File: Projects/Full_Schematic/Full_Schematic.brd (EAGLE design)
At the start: 100 x 69 mm, 79 parts, among them J1 10118193-0001LF, Q1 SS8050-G, Q2 SS8050-G, SW1 OS102011MS2QN1, SW2 OS102011MS2QN1, U1 LM324, U10 SC189ZSKTRT, U2 ACS70331EESATR-005U3, U3 74HC4051PW,118, U4 NA555DR, U5 FT260Q-T, U6 MIC5387-SGFYMT-TR, U7 ESP32-WROOM-32E_(16MB), U8 SCD41-D-R1, U9 HDC1080DMBR

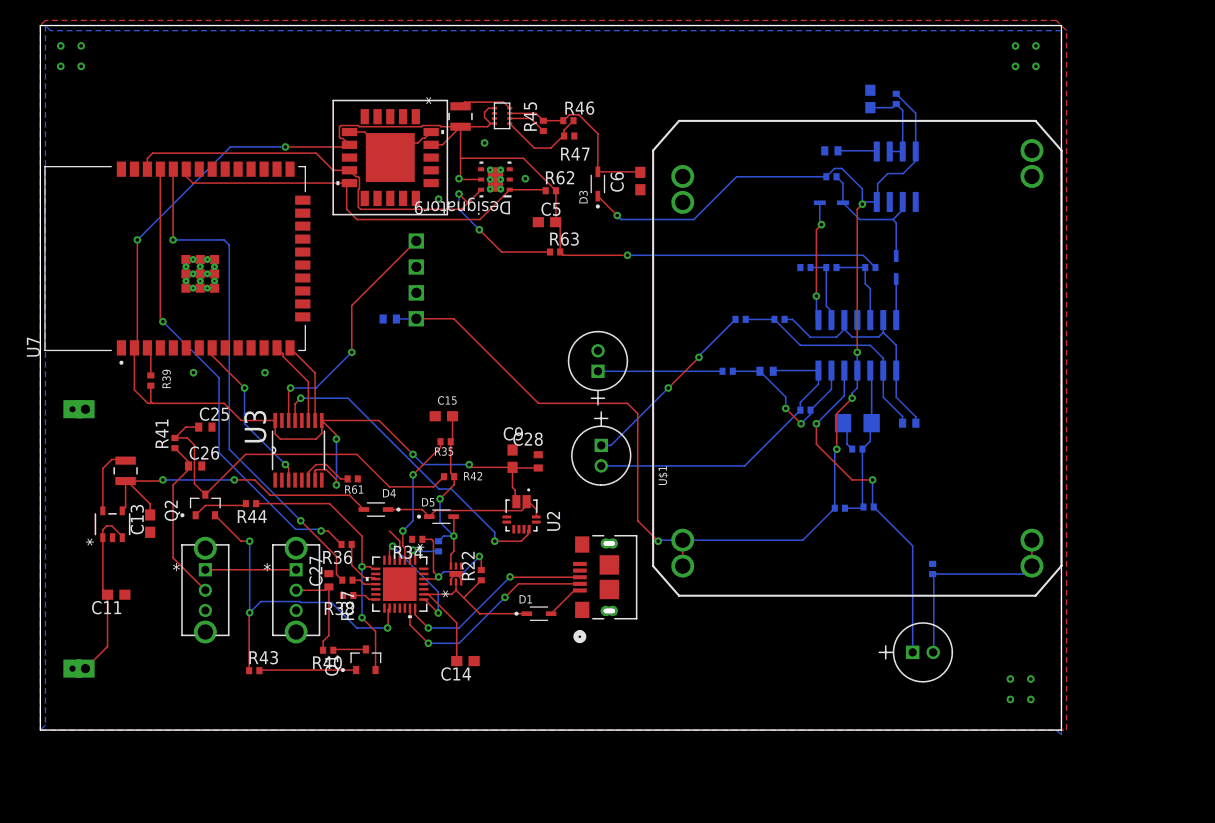
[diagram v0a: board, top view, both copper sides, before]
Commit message: Final revision of the Full Schematic, haven't updated in a while since I was soloing this one.
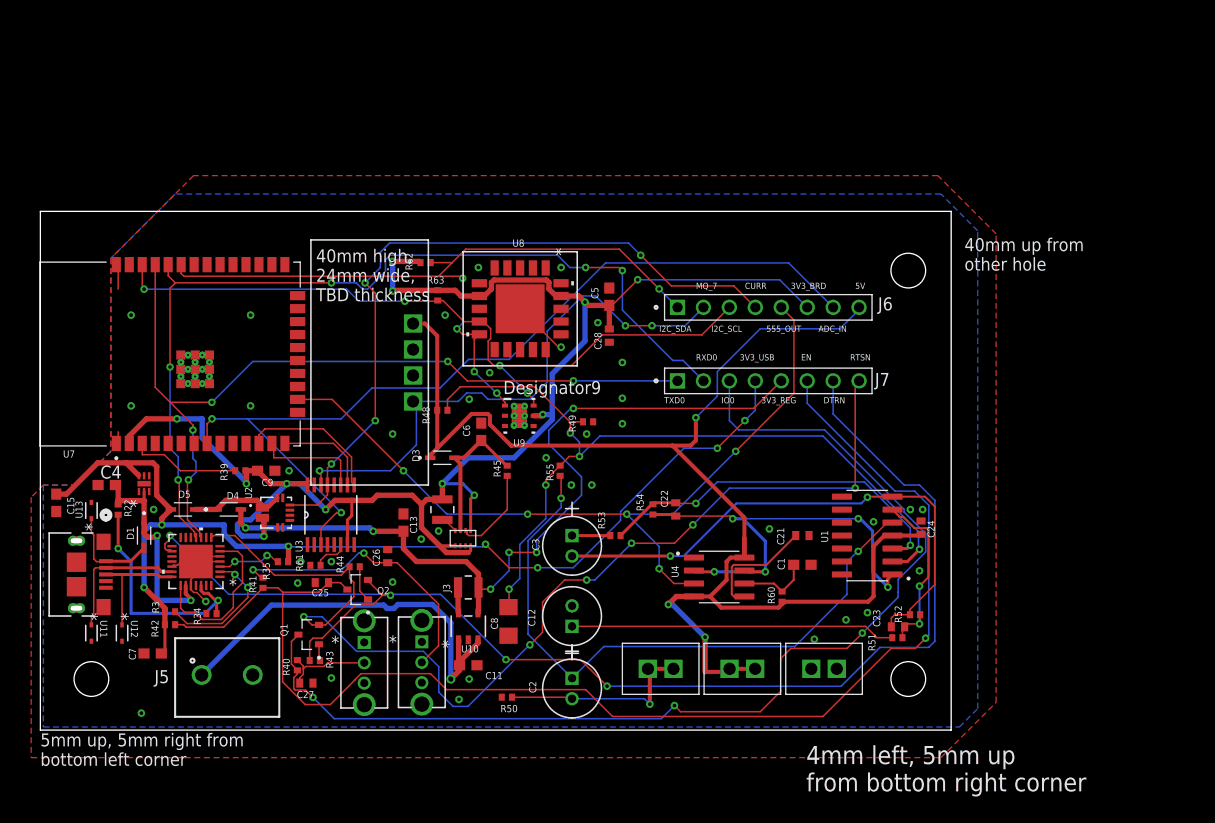
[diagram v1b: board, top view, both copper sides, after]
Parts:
- removed C14: 22uF, rcl:C0603
- removed CR1, CR2: 1N4148WX-TP, 1n4148WX-TP_Diode:CR_SOD323_MCC
- removed R36, R37, R38, R47: 10k, rcl:R0402
- removed R46: 73k, rcl:R0402
- removed R56: 680k, rcl:R0402
- removed R57: 50k, rcl:R0402
- removed R58, R59: 1M, rcl:R0402
- added C4, C7: 1uF, rcl:C0603
- added J5: 691137710002, 691137710002:691137710002
- added J6, J7: 826629-8, 826629-8:TE_826629-8
- added U$5: 2PIN_HEADER, 2PIN_HEADER:2PIN_HEADER
- added U11, U12, U13: ESD5Z5.0T1G, Circuit_protection_diode:SOD-523_0P9X1P3_ONS
- U$1: value HB100 -> 2PIN_HEADER; device HB100_Doppler:HB100 -> 2PIN_HEADER:2PIN_HEADER
- U$2: value POWER_CONN -> 2PIN_HEADER; device PWR_IN:POWER_CONN -> 2PIN_HEADER:2PIN_HEADER
- moved U$2 65.9 mm to (67.5, 6.00), turned to 180 degrees
- moved C24 55.9 mm to (86.2, 19.8), flipped to the top, turned to 270 degrees
- moved J1 51.6 mm to (3.81, 15.2), turned to 270 degrees
- moved R60 50.0 mm to (72.6, 13.1), flipped to the top, turned to 270 degrees
- moved C1 46.1 mm to (74.6, 16.2), flipped to the top, turned to 0 degrees
- moved R50 43.5 mm to (45.7, 3.22), flipped to the top, turned to 0 degrees
- moved U4 42.9 mm to (66.5, 15.0), flipped to the top, turned to 0 degrees
- moved U$4 42.1 mm to (40.6, 19.1), turned to 90 degrees
- moved R48 40.1 mm to (39.4, 31.3), flipped to the top, turned to 180 degrees
- moved D1 39.4 mm to (10.2, 19.1), turned to 270 degrees
- moved C8 39.3 mm to (45.9, 10.6), flipped to the top, turned to 270 degrees
- moved C15 38.9 mm to (1.56, 22.3), turned to 90 degrees
- moved L4 38.5 mm to (39.4, 21.6), turned to 90 degrees
- moved C21 37.8 mm to (74.6, 19.1), flipped to the top
- moved U10 36.2 mm to (41.9, 10.2)
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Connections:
- removed net N$1: C2.2, R50.2, U$1.IF@1, U$1.IF@2
- removed net N$11: R56.1, R57.2, U1.12
- removed net N$15: CR1.1, U1.8
- removed net N$17: CR1.2, CR2.2, R59.1, U4.2
- removed net N$18: CR2.1, U1.14
- removed net N$36: U7.16
- removed net N$48: U7.12
- removed net N$58: R46.1, R47.2, U$4.8
- removed net N$61: R57.1, R58.2, U1.9
- removed net RXD: R36.1, U5.10
- removed net TO_DISC_IN: U4.3
- removed net TXD: R37.1, U5.11
- new net 555_OUT: J6.5, U4.3, U7.16
- new net D3: U3.9, U7.12
- new net N$29: C2.2, R50.2, U$1.1, U$1.2
- net 3V3_BRD: now also J6.6, U$4.8; no longer R56.2, U3.9
- net 3V3_EXT: now also J5.1; no longer U$2.1, U$2.3
- net 3V3_REG: now also J7.5
- net 3V3_USB: now also C7.2, J7.4
- net 5V: now also J6.8, U$2.1, U$2.2; no longer R59.2, U$1.5V@1, U$1.5V@2
- net 5V1: no longer R46.2
- net 5V_EXT: now also C4.2; no longer C14.2
- net ADC_IN: now also J6.7
- net DTRN: now also J7.7
- net EN: now also J7.6
- net GND: now also C4.1, C7.1, J5.2, U$5.1, U$5.2, U11.2, U12.2, U13.2; no longer C14.1, R38.2, R47.1, R58.1, U$1.GND@1, U$1.GND@2, U$1.GND@3, U$1.GND@4, U$2.2, U$2.4
- net I2C_SCL: now also J6.3
- net I2C_SDA: now also J6.1
- net IO0: now also J7.3
- net N$16: now also J6.2
- net N$20: now also U13.1
- net N$22: now also U11.1
- net N$23: now also U12.1
- net N$6: now also U1.3; no longer U1.2
- net N$7: now also J6.4
- net N$8: now also C1.1, R60.1, U4.6; no longer C22.2, R54.2, U1.1, U1.10, U1.13
- net N$9: now also U1.2; no longer U1.3
- net RTSN: now also J7.8
- net RXD0: now also J7.2, U5.11; no longer R37.2
- net SUSPENDN: no longer R38.1
- net THRESH_NET: now also C22.2, R54.2, U1.1, U4.2; no longer C1.1, R60.1, U4.6
- net TXD0: now also J7.1, U5.10; no longer R36.2
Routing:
- net IO0: track 3.22 -> 108.9 mm, vias 0 -> 3
- net DTRN: track 34.2 -> 129.7 mm, vias 3 -> 4
- net EN: track 37.3 -> 129.8 mm, vias 0 -> 1
- net 3V3_USB: track 19.8 -> 106.7 mm, vias 2 -> 7
- net RTSN: track 26.8 -> 105.4 mm, vias 2 -> 6
- net 555_OUT: track 0.00 -> 77.7 mm, vias 0 -> 5
- net ADC_IN: track 16.1 -> 88.8 mm
- net N$9: track 15.7 -> 81.3 mm, vias 0 -> 5
- net 3V3_REG: track 31.9 -> 79.7 mm, vias 2 -> 6
- net RXD0: track 50.1 -> 89.6 mm, vias 2 -> 5
- net N$7: track 31.8 -> 70.6 mm, vias 2 -> 4
- net THRESH_NET: track 8.87 -> 45.8 mm, vias 0 -> 5
- net TXD0: track 45.9 -> 81.4 mm, vias 2 -> 5
- net I2C_SDA: track 40.9 -> 73.6 mm, vias 0 -> 5
- net N$16: track 24.2 -> 54.5 mm, vias 2 -> 3
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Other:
- board size 100 x 69 mm -> 89.2 x 50.8 mm
- board text added: "3V3_BRD"
- board text added: "3V3_REG"
- board text added: "3V3_USB"
- board text added: "40mm high, 24mm wide, TBD thickness"
- board text added: "40mm up from other hole"
- board text added: "4mm left, 5mm up from bottom right corner"
- board text added: "555_OUT"
- board text added: "5V"
- board text added: "5mm up, 5mm right from bottom left corner"
- board text added: "ADC_IN"
- board text added: "BS"
- board text added: "CURR"
- board text added: "DTRN"
- board text added: "EN"
- board text added: "I2C_SCL"
- board text added: "I2C_SDA"
- board text added: "IO0"
- board text added: "MQ_7"
- board text added: "RTSN"
- board text added: "RXD0"
- board text added: "TXD0"
- board text added: "YCP"
